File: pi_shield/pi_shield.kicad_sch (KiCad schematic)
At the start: 33 parts, among them J1 PUMP_NUTRI, J10 1_WIRE, J11 TDS, J12 pH, J2 PUMP_WATER, J3 CLOSURE_WATER, J4 CLOSURE_NUTRI, J5 LEVEL_WATER, J6 LEVEL_NUTRI, J7 Raspberry_Pi_2_3, J8 POWER, J9 12V OUT, Q1 Q_NMOS_DGS, Q2 Q_NMOS_DGS, SW1 NUTRI_ENA, SW2 WATER_ENA, U1 ATtiny85-20P

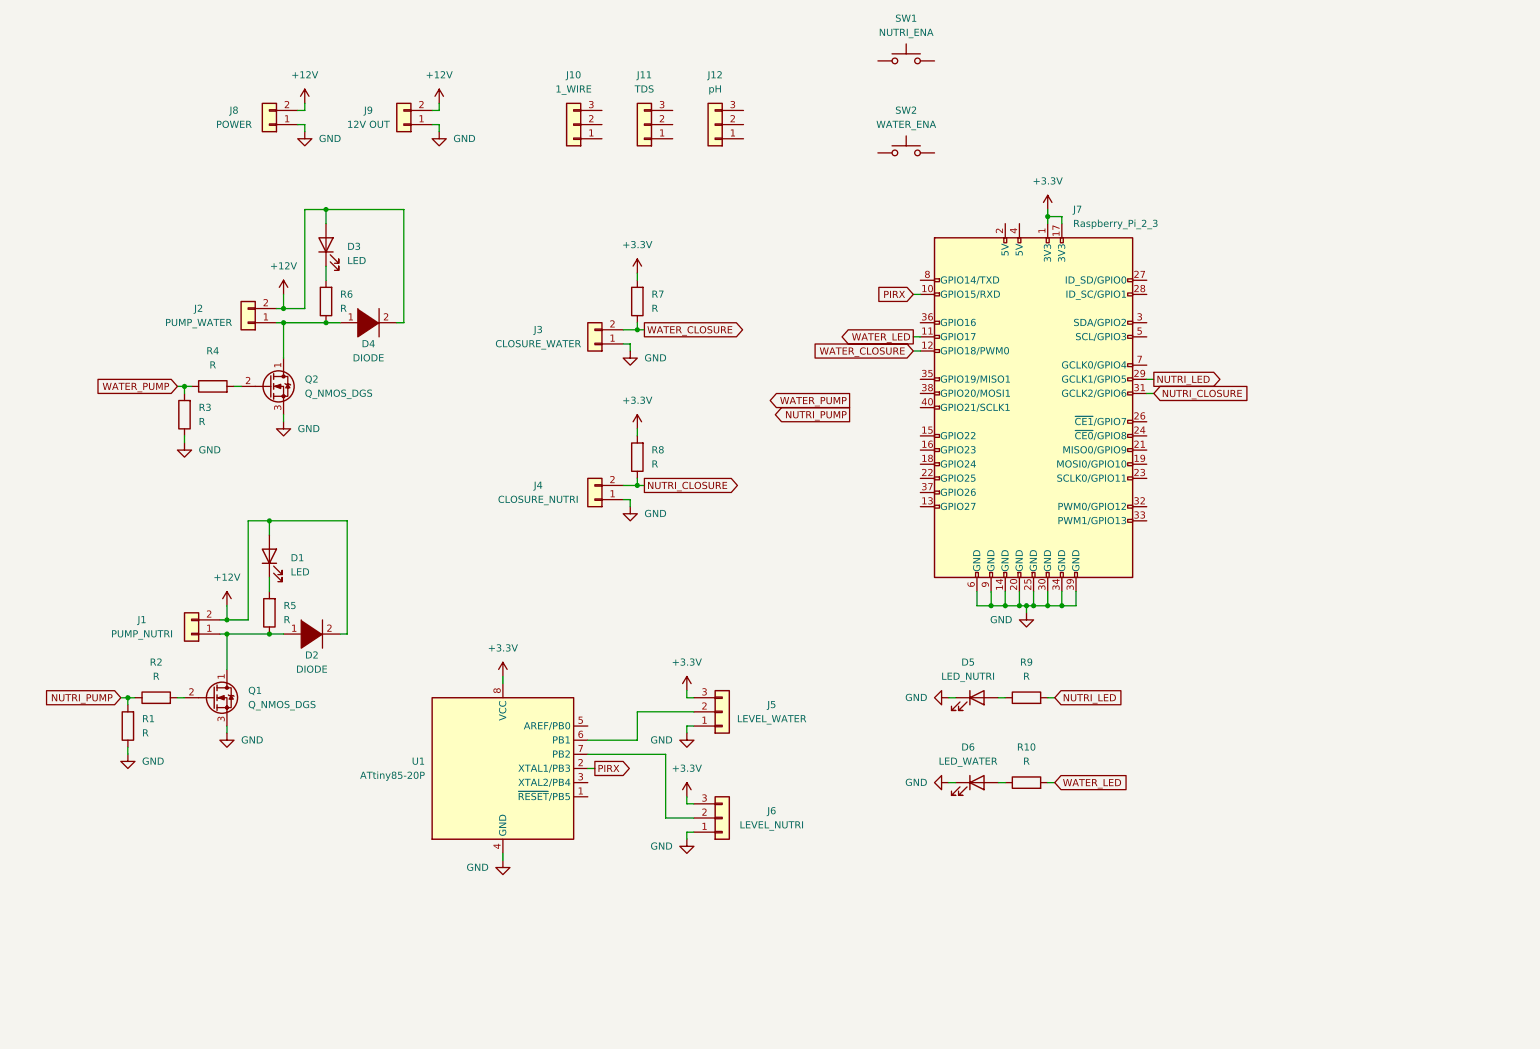
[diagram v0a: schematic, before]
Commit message: Finish PCBs
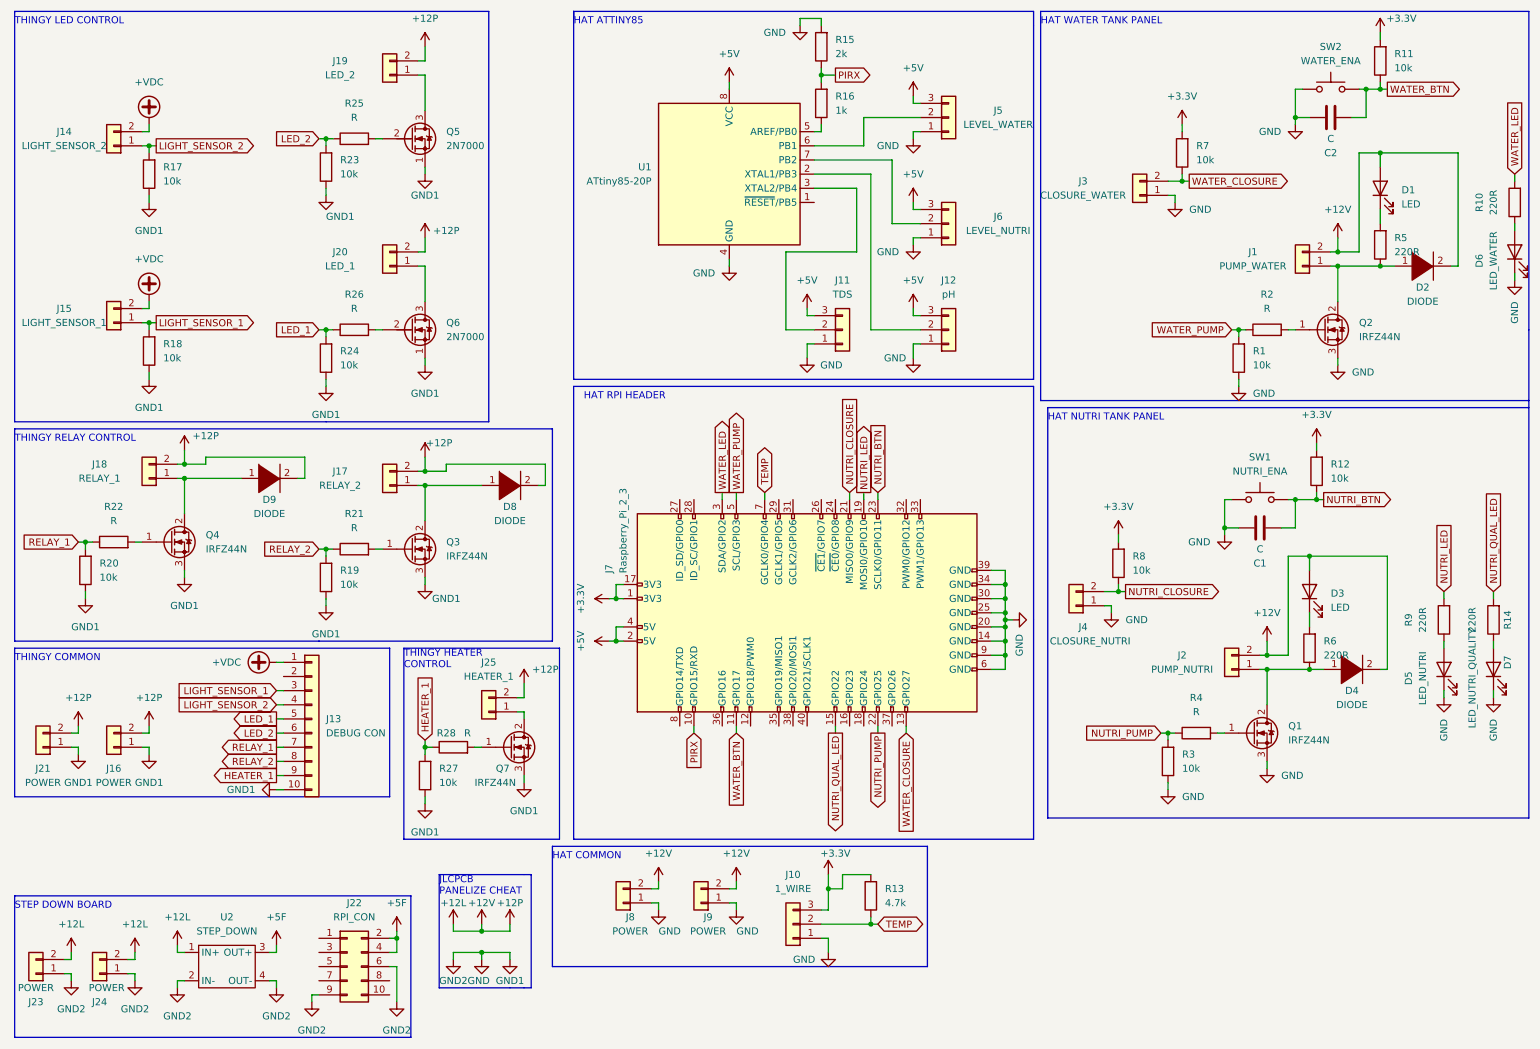
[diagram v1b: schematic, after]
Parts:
- removed Q1, Q2: Q_NMOS_DGS, symbol Device:Q_NMOS_DGS
- added C1, C2: C, Capacitor_THT:C_Disc_D5.0mm_W2.5mm_P2.50mm, symbol Device:C
- added D7: LED_NUTRI_QUALITY, LED_THT:LED_D5.0mm_Clear, symbol Device:LED
- added D8, D9: DIODE, Diode_THT:D_A-405_P2.54mm_Vertical_AnodeUp, symbol pspice:DIODE
- added J13: DEBUG CON, Connector_PinSocket_2.54mm:PinSocket_1x10_P2.54mm_Vertical, symbol Connector_Generic:Conn_01x10
- added J14: LIGHT_SENSOR_2, Connector_Molex:Molex_SL_171971-0002_1x02_P2.54mm_Vertical, symbol Connector_Generic:Conn_01x02
- added J15: LIGHT_SENSOR_1, Connector_Molex:Molex_SL_171971-0002_1x02_P2.54mm_Vertical, symbol Connector_Generic:Conn_01x02
- added J16, J21, J23, J24: POWER, Connector_Molex:Molex_SL_171971-0002_1x02_P2.54mm_Vertical, symbol Connector_Generic:Conn_01x02
- added J17: RELAY_2, Connector_Molex:Molex_SL_171971-0002_1x02_P2.54mm_Vertical, symbol Connector_Generic:Conn_01x02
- added J18: RELAY_1, Connector_Molex:Molex_SL_171971-0002_1x02_P2.54mm_Vertical, symbol Connector_Generic:Conn_01x02
- added J19: LED_2, Connector_Molex:Molex_SL_171971-0002_1x02_P2.54mm_Vertical, symbol Connector_Generic:Conn_01x02
- added J20: LED_1, Connector_Molex:Molex_SL_171971-0002_1x02_P2.54mm_Vertical, symbol Connector_Generic:Conn_01x02
- added J22: RPI_CON, Connector_PinSocket_2.54mm:PinSocket_2x05_P2.54mm_Vertical, symbol Connector_Generic:Conn_02x05_Odd_Even
- added J25: HEATER_1, Connector_Molex:Molex_SL_171971-0002_1x02_P2.54mm_Vertical, symbol Connector_Generic:Conn_01x02
- added Q1, Q2, Q7: IRFZ44N, Package_TO_SOT_THT:TO-220-3_Horizontal_TabDown, symbol Device:Q_NMOS_GDS
- added Q3, Q4: IRFZ44N, Package_TO_SOT_THT:TO-220-3_Vertical, symbol Device:Q_NMOS_GDS
- added Q5, Q6: 2N7000, Package_TO_SOT_THT:TO-92L_Inline, symbol Device:Q_NMOS_SGD
- added R11, R12, R17, R18, R19, R20, R23, R24, R27: 10k, Resistor_THT:R_Axial_DIN0204_L3.6mm_D1.6mm_P2.54mm_Vertical, symbol Device:R
- added R13: 4.7k, Resistor_THT:R_Axial_DIN0204_L3.6mm_D1.6mm_P2.54mm_Vertical, symbol Device:R
- added R14: 220R, Resistor_THT:R_Axial_DIN0204_L3.6mm_D1.6mm_P2.54mm_Vertical, symbol Device:R
- added R15: 2k, Resistor_THT:R_Axial_DIN0204_L3.6mm_D1.6mm_P2.54mm_Vertical, symbol Device:R
- added R16: 1k, Resistor_THT:R_Axial_DIN0204_L3.6mm_D1.6mm_P2.54mm_Vertical, symbol Device:R
- added R21, R22, R25, R26, R28: R, Resistor_THT:R_Axial_DIN0204_L3.6mm_D1.6mm_P2.54mm_Vertical, symbol Device:R
- added U2: STEP_DOWN, Custom:SRT_MPT1584EN_Module, symbol Custom:STEP_DOWN
- J1: value PUMP_NUTRI -> PUMP_WATER
- J2: value PUMP_WATER -> PUMP_NUTRI
- J9: value 12V OUT -> POWER
- R1, R3, R7, R8: value R -> 10k
- R10, R5, R6, R9: value R -> 220R
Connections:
- net +3.3V: now also J10.3 (Pin_3), R11.2, R12.2, R13.2; no longer J5.3 (Pin_3), J6.3 (Pin_3), U1.8 (VCC)
- net GND: now also J10.1 (Pin_1), J11.1 (Pin_1), J12.1 (Pin_1), SW1.1, SW2.1, C1.1, C2.1, D7.1 (K), J13.10 (Pin_10), J16.1 (Pin_1), J21.1 (Pin_1), J22.6 (Pin_6), J22.9 (Pin_9), J23.1 (Pin_1), J24.1 (Pin_1), Q1.3 (S), Q2.3 (S), Q3.3 (S), Q4.3 (S), Q5.1 (S), Q6.1 (S), Q7.3 (S), R15.2, R17.1, R18.1, R19.1, R20.1, R23.1, R24.1, R27.1, U2.2 (IN-), U2.4 (OUT-)
- net NUTRI_CLOSURE: now also J7.21 (MISO0/GPIO9); no longer J7.31 (GCLK2/GPIO6)
- net NUTRI_LED: now also J7.19 (MOSI0/GPIO10); no longer J7.29 (GCLK1/GPIO5)
- net NUTRI_PUMP: now also J7.22 (GPIO25), R3.2, R4.1; no longer R1.2, R2.1
- net PIRX: now also R15.1, R16.2; no longer U1.2 (XTAL1/PB3)
- net WATER_CLOSURE: now also J7.13 (GPIO27); no longer J7.12 (GPIO18/PWM0)
- net WATER_LED: now also J7.3 (SDA/GPIO2); no longer J7.11 (GPIO17)
- net WATER_PUMP: now also J7.5 (SCL/GPIO3), R1.2, R2.1; no longer R3.2, R4.1
- net TEMP: now reaches J10.2 (Pin_2)
- net TEMP: now also J7.7 (GCLK0/GPIO4), R13.1
- net at J12.2 (Pin_2): now also U1.2 (XTAL1/PB3)
- net +5V: now reaches J12.3 (Pin_3)
- net +5V: now also J11.3 (Pin_3), J5.3 (Pin_3), J6.3 (Pin_3), J7.2 (5V), J7.4 (5V), U1.8 (VCC)
- net at D2.1 (K), J1.1 (Pin_1), R5.1: now also Q2.2 (D)
- net at U1.3 (XTAL2/PB4): now also J11.2 (Pin_2)
- net at U1.5 (AREF/PB0): now also R16.1
- net NUTRI_BTN: now reaches SW1.2
- net NUTRI_BTN: now also J7.23 (SCLK0/GPIO11), C1.2, R12.1
- net WATER_BTN: now reaches SW2.2
- net WATER_BTN: now also J7.11 (GPIO17), C2.2, R11.1
- net at R2.2: now also Q2.1 (G)
- net at R4.2: now also Q1.1 (G)
- net at D4.1 (K), J2.1 (Pin_1), R6.1: now also Q1.2 (D)
- net NUTRI_QUAL_LED: now reaches J7.15 (GPIO22)
- net NUTRI_QUAL_LED: now also R14.2
- net +12V renamed +12L
- net +12L: now also D8.2 (A), D9.2 (A), J16.2 (Pin_2), J17.2 (Pin_2), J18.2 (Pin_2), J19.2 (Pin_2), J20.2 (Pin_2), J21.2 (Pin_2), J23.2 (Pin_2), J24.2 (Pin_2), J25.2 (Pin_2), U2.1 (IN+)
- new net: Q3.1 (G), R21.2
- new net: D9.1 (K), J18.1 (Pin_1), Q4.2 (D)
- new net: J20.1 (Pin_1), Q6.3 (D)
- new net: D7.2 (A), R14.1
- new net: D8.1 (K), J17.1 (Pin_1), Q3.2 (D)
- new net: J25.1 (Pin_1), Q7.2 (D)
- new net: Q4.1 (G), R22.2
- new net: Q5.2 (G), R25.2
- new net: Q7.1 (G), R28.2
- new net: Q6.2 (G), R26.2
- new net: J19.1 (Pin_1), Q5.3 (D)
- new net +5F: J22.2 (Pin_2), J22.4 (Pin_4), U2.3 (OUT+)
- new net +VDC: J13.1 (Pin_1), J14.2 (Pin_2), J15.2 (Pin_2)
- new net HEATER_1: J13.9 (Pin_9), R27.2, R28.1
- new net LED_1: J13.5 (Pin_5), R24.2, R26.1
- new net LED_2: J13.6 (Pin_6), R23.2, R25.1
- new net LIGHT_SENSOR_1: J13.3 (Pin_3), J15.1 (Pin_1), R18.2
- new net LIGHT_SENSOR_2: J13.4 (Pin_4), J14.1 (Pin_1), R17.2
- new net RELAY_1: J13.7 (Pin_7), R20.2, R22.1
- new net RELAY_2: J13.8 (Pin_8), R19.2, R21.1
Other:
- note added: "HAT ATTINY85"
- note added: "HAT COMMON"
- note added: "HAT NUTRI TANK PANEL"
- note added: "HAT RPI HEADER"
- note added: "HAT WATER TANK PANEL"
- note added: "JLCPCB PANELIZE CHEAT"
- note added: "STEP DOWN BOARD"
- note added: "THINGY COMMON"
- note added: "THINGY HEATER CONTROL"
- note added: "THINGY LED CONTROL"
- note added: "THINGY RELAY CONTROL"
- moved on the sheet: D1, D2, D3, D4, D5, D6, J1, J10, J11, J12, J2, J3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
